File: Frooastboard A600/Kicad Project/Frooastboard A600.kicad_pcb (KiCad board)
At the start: 2 copper layers, 319.1 x 128.6 mm, 207 parts, among them J1 PS2_5V, J3 SW Interface, J8 USB, Q1 BSS138, Q2 BSS138, U2 RP2040, U3 W25Q32JVZP, U4 LM317L_SOT-89, Y1 12MHz

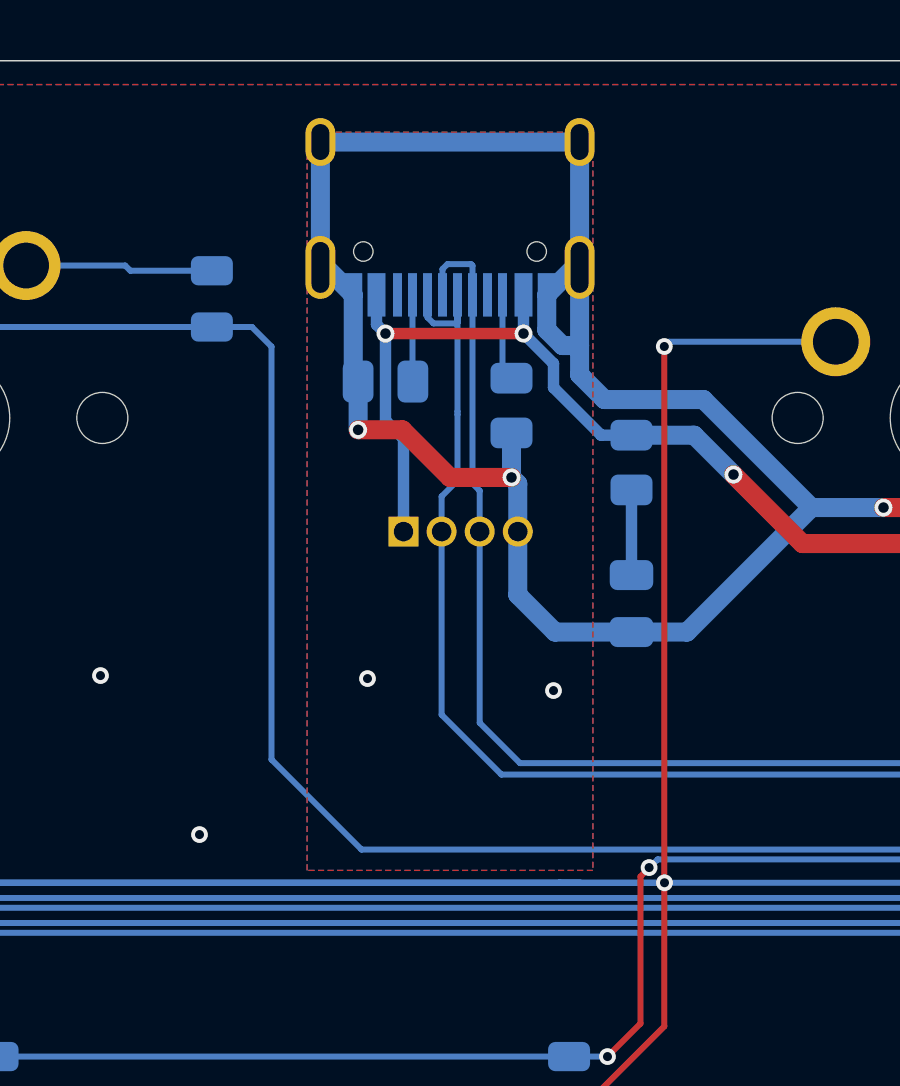
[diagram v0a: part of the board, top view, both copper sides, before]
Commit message: prepare for pcba
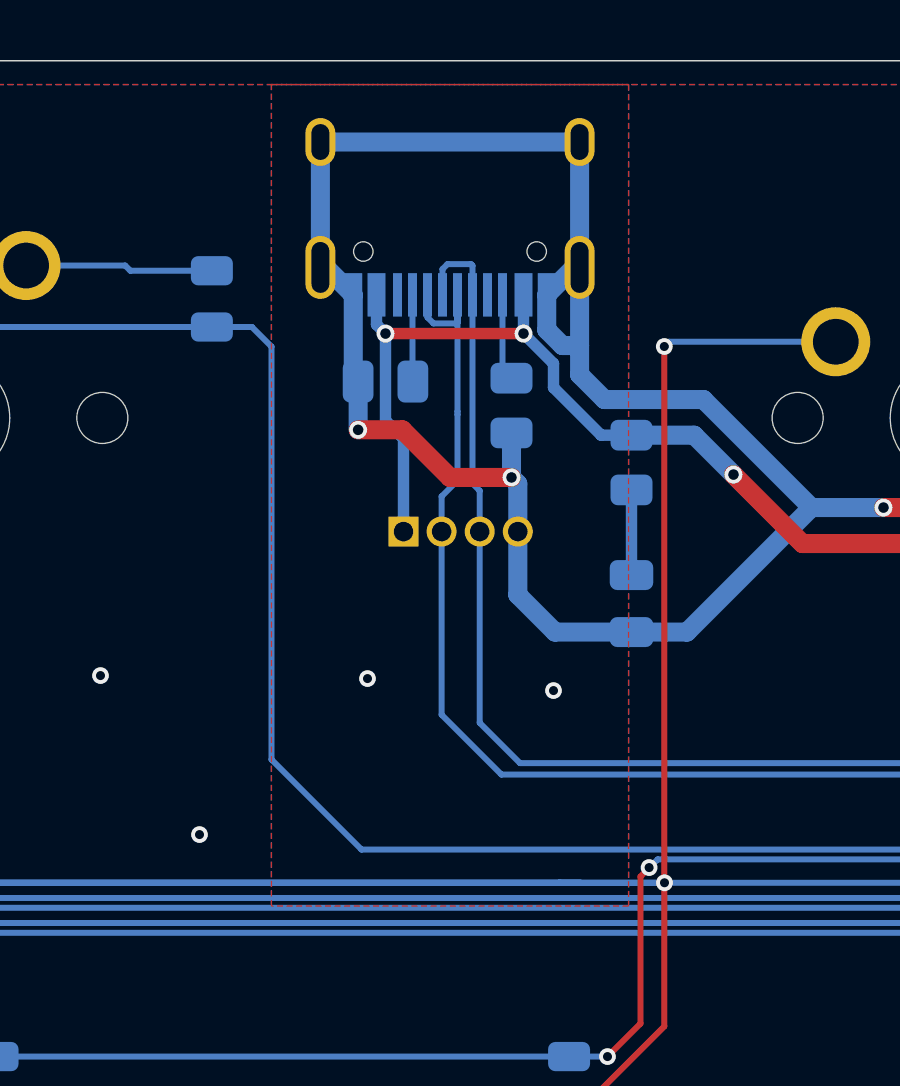
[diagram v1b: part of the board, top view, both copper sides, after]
